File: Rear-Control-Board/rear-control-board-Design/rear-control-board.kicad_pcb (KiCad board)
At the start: 2 copper layers, 139.1 x 102.8 mm, 55 parts, among them J1 Conn_01x23, J2 Conn_01x23, J3 Conn_01x08, J4 JST-B2B-VERT-2PIN, J5 JST-B2B-VERT-2PIN, J6 Conn_01x02, J7 Micro_SD_Card, K1 T9VV1K15-12S, K2 G5V-2, K3 G5V-2, Q2 PSMN5R2-60YL, Q3 PSMN5R2-60YL, Q4 PSMN5R2-60YL, U1 Dev_Board_C, U2 TS2940CP33 ROG, U4 MAX33054EASA+T

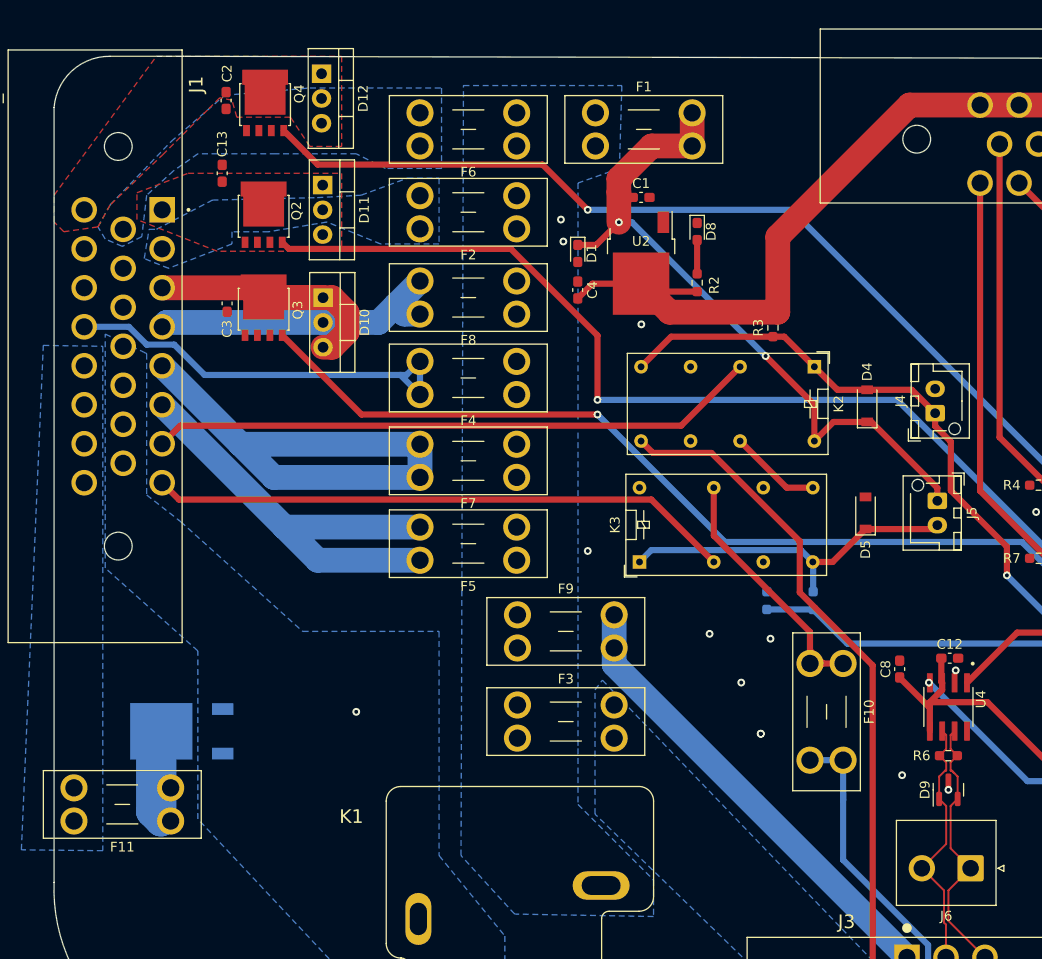
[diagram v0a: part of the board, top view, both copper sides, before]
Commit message: V1 with all Gerbers
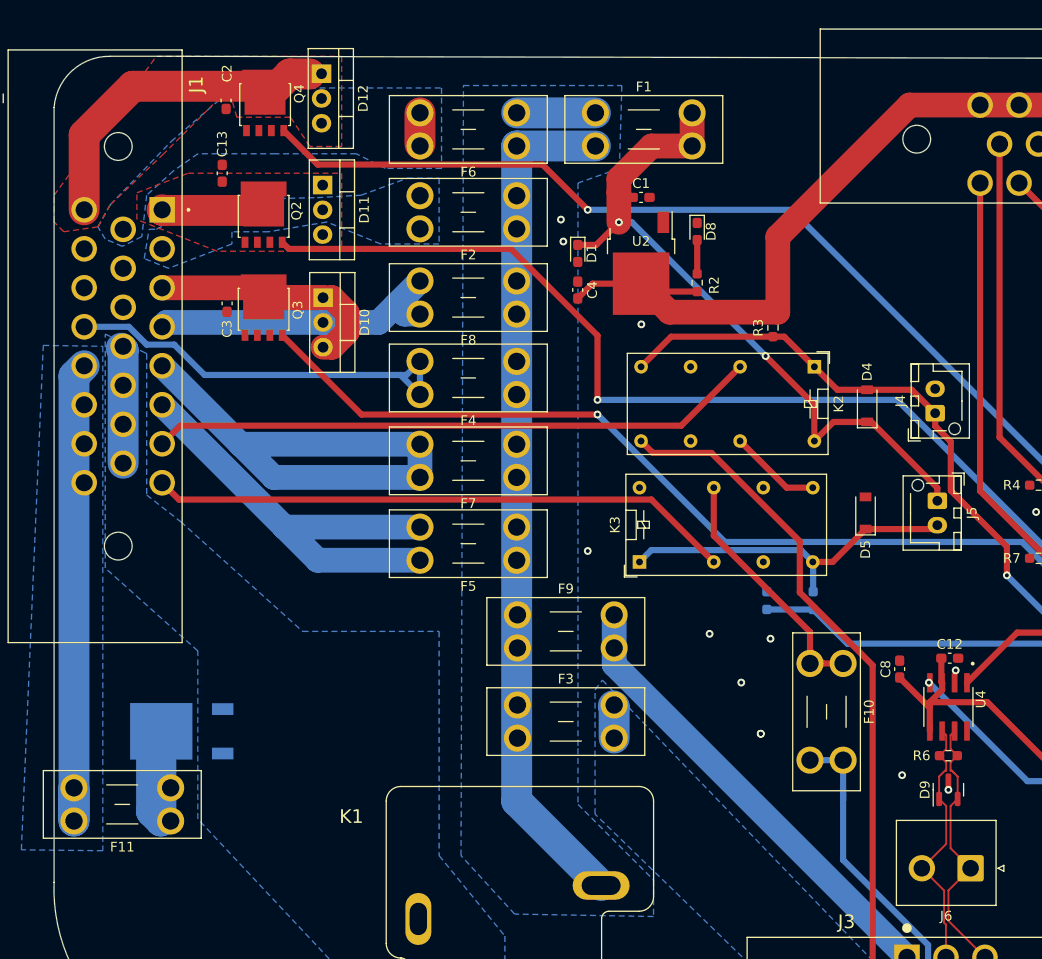
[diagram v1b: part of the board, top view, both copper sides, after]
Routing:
- net +12V: track 0.00 -> 95.6 mm
- net /DCDC_IN: track 0.00 -> 50.5 mm
- net /PUMP_RTRN_12V: track 0.00 -> 34.5 mm
- net /FAN_RTRN_12V: track 0.00 -> 12.4 mm
- net /BATT_12V: track 0.00 -> 11.9 mm
- net /RINE_12: track 0.00 -> 3.35 mm
- net /PUMP_12V: track 0.00 -> 3.20 mm
- net GND: vias 17 -> 16
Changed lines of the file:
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@@
       (drillshape 0)
       (scaleselection 1)
-      (outputdirectory "RCB_Gerber/")
+      (outputdirectory "../../BOARD GERBER/V1/RCB/")
     )
   )
@@
     (fp_line (start -2.45 3.4) (end 4.95 3.4) (layer "F.Fab") (width 0.1))
     (pad "" np_thru_hole circle (at -1.6 2 90) (size 1.2 1.2) (drill 1.2) (layers *.Cu *.Mask))
-    (pad "1" thru_hole roundrect (at 0 0 90) (size 1.7 2) (drill 1) (layers *.Cu *.Mask) (roundrect_rratio 0.147059)
+    (pad "1" thru_hole roundrect (at 0 0 90) (size 1.7 2) (drill 1) (layers *.Cu *.Mask) (roundrect_rratio 0.1470588235)
       (net 67 "/FAULT_LATCHER/BMS_SWITCH") (pinfunction "Pin_1") (pintype "passive"))
     (pad "2" thru_hole oval (at 2.5 0 90) (size 1.7 2) (drill 1) (layers *.Cu *.Mask)
@@
     (fp_line (start -2.45 3.4) (end 4.95 3.4) (layer "F.Fab") (width 0.1))
     (pad "" np_thru_hole circle (at -1.6 2 270) (size 1.2 1.2) (drill 1.2) (layers *.Cu *.Mask))
-    (pad "1" thru_hole roundrect (at 0 0 270) (size 1.7 2) (drill 1) (layers *.Cu *.Mask) (roundrect_rratio 0.147059)
+    (pad "1" thru_hole roundrect (at 0 0 270) (size 1.7 2) (drill 1) (layers *.Cu *.Mask) (roundrect_rratio 0.1470588235)
       (net 3 "INT_12V") (pinfunction "Pin_1") (pintype "passive"))
     (pad "2" thru_hole oval (at 2.5 0 270) (size 1.7 2) (drill 1) (layers *.Cu *.Mask)
@@
     (fp_line (start -2.5 -3.7) (end -2.5 4.8) (layer "F.Fab") (width 0.1))
     (fp_line (start -2.5 -1) (end -1.5 0) (layer "F.Fab") (width 0.1))
-    (pad "1" thru_hole roundrect (at 0 0 180) (size 2.7 2.7) (drill 1.7) (layers *.Cu *.Mask) (roundrect_rratio 0.092593)
+    (pad "1" thru_hole roundrect (at 0 0 180) (size 2.7 2.7) (drill 1.7) (layers *.Cu *.Mask) (roundrect_rratio 0.09259296296)
       (net 19 "/CAN_P") (pinfunction "Pin_1") (pintype "passive"))
     (pad "2" thru_hole circle (at 5 0 180) (size 2.7 2.7) (drill 1.7) (layers *.Cu *.Mask)
@@
   (via (at 190.5 153) (size 0.8) (drill 0.4) (layers "F.Cu" "B.Cu") (free) (net 1))
   (via (at 131 131) (size 0.8) (drill 0.4) (layers "F.Cu" "B.Cu") (free) (net 1))
-  (via (at 89.5 128.75) (size 0.8) (drill 0.4) (layers "F.Cu" "B.Cu") (free) (net 1))
   (via (at 110.5 78.25) (size 0.8) (drill 0.4) (layers "F.Cu" "B.Cu") (free) (net 1))
   (via (at 177.5 128.75) (size 0.8) (drill 0.4) (layers "F.Cu" "B.Cu") (free) (net 1))
@@
   (via (at 113.25 112.25) (size 0.8) (drill 0.4) (layers "F.Cu" "B.Cu") (free) (net 1))
   (via (at 150.25 136.75) (size 0.8) (drill 0.4) (layers "F.Cu" "B.Cu") (free) (net 1))
+  (segment (start 80.15 65.85) (end 78.87298 64.57298) (width 3.175) (layer "F.Cu") (net 2))
+  (segment (start 82.689297 63.310703) (end 84.748777 63.315161) (width 3.175) (layer "F.Cu") (net 2))
+  (segment (start 61.5875 69.566094) (end 61.5875 77.25) (width 3.175) (layer "F.Cu") (net 2))
+  (segment (start 80.15 65.85) (end 82.689297 63.310703) (width 3.175) (layer "F.Cu") (net 2))
+  (segment (start 78.87298 64.57298) (end 66.580614 64.57298) (width 3.175) (layer "F.Cu") (net 2))
+  (segment (start 66.580614 64.57298) (end 61.5875 69.566094) (width 3.175) (layer "F.Cu") (net 2))
   (segment (start 117.8625 75.975) (end 116.975 75.975) (width 0.635) (layer "F.Cu") (net 3))
   (segment (start 141.9175 99.013615) (end 138.4575 99.013615) (width 0.635) (layer "F.Cu") (net 3))
@@
   (segment (start 131.5 92.25) (end 117.775 78.525) (width 0.635) (layer "B.Cu") (net 3))
   (segment (start 117.775 78.525) (end 116.445 78.525) (width 0.635) (layer "B.Cu") (net 3))
+  (segment (start 105.96 137.905) (end 114.625 146.57) (width 3.175) (layer "B.Cu") (net 4))
+  (segment (start 105.96 70.7) (end 105.96 137.905) (width 3.175) (layer "B.Cu") (net 4))
+  (segment (start 114.04 70.7) (end 105.96 70.7) (width 3.175) (layer "B.Cu") (net 4))
+  (segment (start 105.96 67.3) (end 114.04 67.3) (width 3.175) (layer "B.Cu") (net 4))
+  (segment (start 65.5875 103.25) (end 65.5875 91.63892) (width 3.175) (layer "B.Cu") (net 6))
+  (segment (start 65.5875 91.63892) (end 65.39304 91.44446) (width 3.175) (layer "B.Cu") (net 6))
   (segment (start 141.75 110.001115) (end 148.7175 110.001115) (width 0.635) (layer "F.Cu") (net 7))
   (segment (start 136.34 113.376115) (end 138.375 113.376115) (width 0.635) (layer "F.Cu") (net 7))
@@
   (segment (start 135.122989 112.159104) (end 119.777011 112.159104) (width 0.635) (layer "B.Cu") (net 7))
   (segment (start 136.375 116.425) (end 136.375 113.411115) (width 0.635) (layer "B.Cu") (net 7))
+  (segment (start 96.04 67.3) (end 96.04 70.502491) (width 3.175) (layer "F.Cu") (net 8))
   (segment (start 96.04 87.95) (end 94.45 87.95) (width 2.54) (layer "B.Cu") (net 9))
   (segment (start 70.0325 88.805) (end 86.095 88.805) (width 2.54) (layer "B.Cu") (net 9))
@@
   (segment (start 80 86.85) (end 80.585 86.265) (width 2.54) (layer "F.Cu") (net 10))
   (segment (start 88.56452 87.801767) (end 87.027753 86.265) (width 2.54) (layer "F.Cu") (net 10))
+  (segment (start 60.54 94.2975) (end 61.5875 93.25) (width 3.175) (layer "B.Cu") (net 11))
+  (segment (start 60.54 139.95) (end 60.54 136.55) (width 3.175) (layer "B.Cu") (net 11))
+  (segment (start 60.54 139.95) (end 60.54 94.2975) (width 3.175) (layer "B.Cu") (net 11))
   (segment (start 69.5875 101.25) (end 71.444511 99.392989) (width 0.635) (layer "F.Cu") (net 12))
   (segment (start 71.444511 99.392989) (end 122.838126 99.392989) (width 0.635) (layer "F.Cu") (net 12))
@@
   (segment (start 149.615 126.491983) (end 149.615 125.775) (width 0.635) (layer "F.Cu") (net 21))
   (segment (start 121.65 87.75) (end 118.725 84.825) (width 2.54) (layer "F.Cu") (net 21))
+  (segment (start 69.6525 77.315) (end 69.5875 77.25) (width 3.175) (layer "F.Cu") (net 22))
+  (segment (start 80 77.315) (end 69.6525 77.315) (width 3.175) (layer "F.Cu") (net 22))
+  (segment (start 80 77.315) (end 78.065 77.315) (width 3.175) (layer "F.Cu") (net 22))
   (segment (start 124.475 80.35) (end 124.475 83.8125) (width 0.635) (layer "F.Cu") (net 23))
   (segment (start 136.05 123.79) (end 136.05 122.45) (width 0.635) (layer "F.Cu") (net 24))
@@
   (segment (start 82.1375 109.8) (end 69.5875 97.25) (width 2.54) (layer "B.Cu") (net 60))
   (segment (start 96.04 113.2) (end 85.5375 113.2) (width 2.54) (layer "B.Cu") (net 60))
+  (segment (start 115.96 131.45) (end 115.96 128.22078) (width 3.175) (layer "B.Cu") (net 62))
+  (segment (start 115.96 128.22078) (end 115.87461 128.13539) (width 3.175) (layer "B.Cu") (net 62))
   (segment (start 115.96 122.2) (end 115.96 123.8975) (width 2.54) (layer "B.Cu") (net 63))
   (segment (start 115.96 123.8975) (end 146 153.9375) (width 2.54) (layer "B.Cu") (net 63))
